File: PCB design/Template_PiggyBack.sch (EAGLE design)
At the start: 46 parts, among them CN1 USB power supply, IC1 MCP6002, IC3 MCP6002, IC4 REG1117

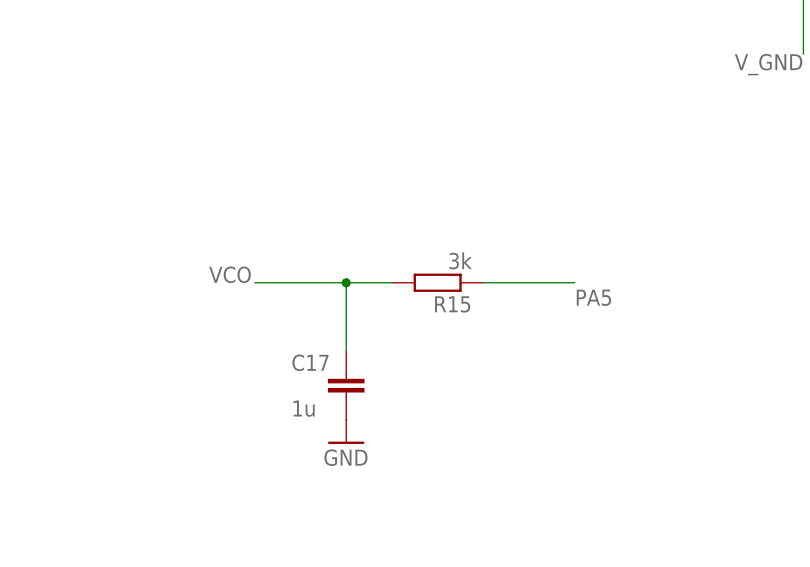
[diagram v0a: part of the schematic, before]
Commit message: finished layout but it is subject to revision
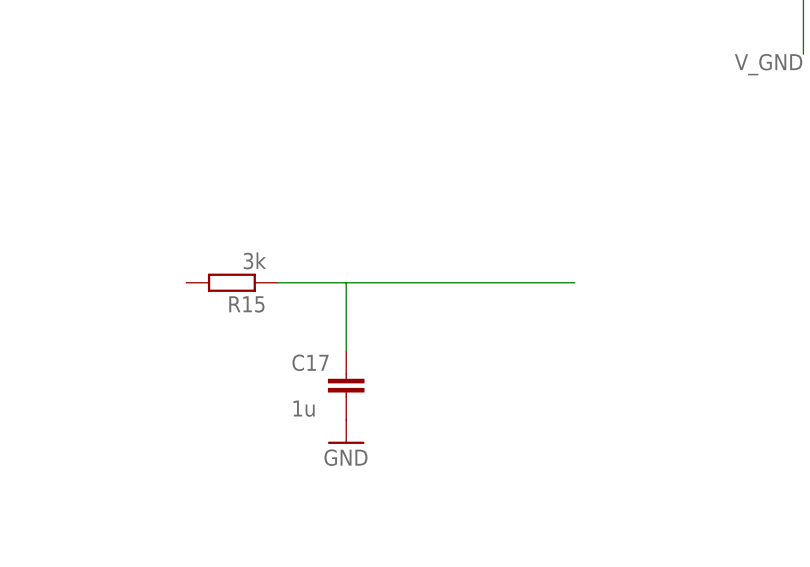
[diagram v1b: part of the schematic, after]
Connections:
- net VCO: no longer R15.2
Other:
- moved on the sheet: R15
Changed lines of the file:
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@@
 <attribute name="VALUE" x="65.024" y="-134.239" size="1.778" layer="96"/>
 </instance>
-<instance part="R15" gate="G$1" x="81.28" y="-119.38" smashed="yes" rot="R180">
-<attribute name="NAME" x="85.09" y="-120.8786" size="1.778" layer="95" rot="R180"/>
-<attribute name="VALUE" x="85.09" y="-116.078" size="1.778" layer="96" rot="R180"/>
+<instance part="R15" gate="G$1" x="58.42" y="-119.38" smashed="yes" rot="R180">
+<attribute name="NAME" x="62.23" y="-120.8786" size="1.778" layer="95" rot="R180"/>
+<attribute name="VALUE" x="62.23" y="-116.078" size="1.778" layer="96" rot="R180"/>
 </instance>
 <instance part="GND1" gate="1" x="71.12" y="-137.16" smashed="yes">
@@
 <segment>
 <pinref part="R15" gate="G$1" pin="1"/>
-<wire x1="86.36" y1="-119.38" x2="96.52" y2="-119.38" width="0.1524" layer="91"/>
-<label x="96.52" y="-121.92" size="1.778" layer="95"/>
+<wire x1="63.5" y1="-119.38" x2="96.52" y2="-119.38" width="0.1524" layer="91"/>
 </segment>
 </net>
@@
 <pinref part="C17" gate="G$1" pin="1"/>
 <wire x1="71.12" y1="-127" x2="71.12" y2="-119.38" width="0.1524" layer="91"/>
-<pinref part="R15" gate="G$1" pin="2"/>
-<wire x1="71.12" y1="-119.38" x2="76.2" y2="-119.38" width="0.1524" layer="91"/>
-<wire x1="71.12" y1="-119.38" x2="60.96" y2="-119.38" width="0.1524" layer="91"/>
-<junction x="71.12" y="-119.38"/>
-<label x="55.88" y="-119.38" size="1.778" layer="95"/>
-</segment>
-</net>
+</segment>
+</net>
